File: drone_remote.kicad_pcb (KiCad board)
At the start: 2 copper layers, 151 x 78.8 mm, 92 parts, among them J1 USBC, J2 Conn_01x02_Socket, J3 UART, J4 Conn_01x05_Pin, J5 Conn_01x04_Socket, J6 Conn_01x08_Socket, J7 Conn_01x09_Socket, J8 Conn_01x09_Socket, Q1 PMOS, SW1 RST_BTN, SW2 RST_BTN, SW3 RST_BTN, SW4 RST_BTN, SW5 RST_BTN, SW6 ENC1, SW7 ENC2, U1 STM32F411RETx, U2 TC1262-33, U3 SN74ALVC14PWR, U4 SN74ALVC14PWR, U6 FT230XS, X1 8MHZ

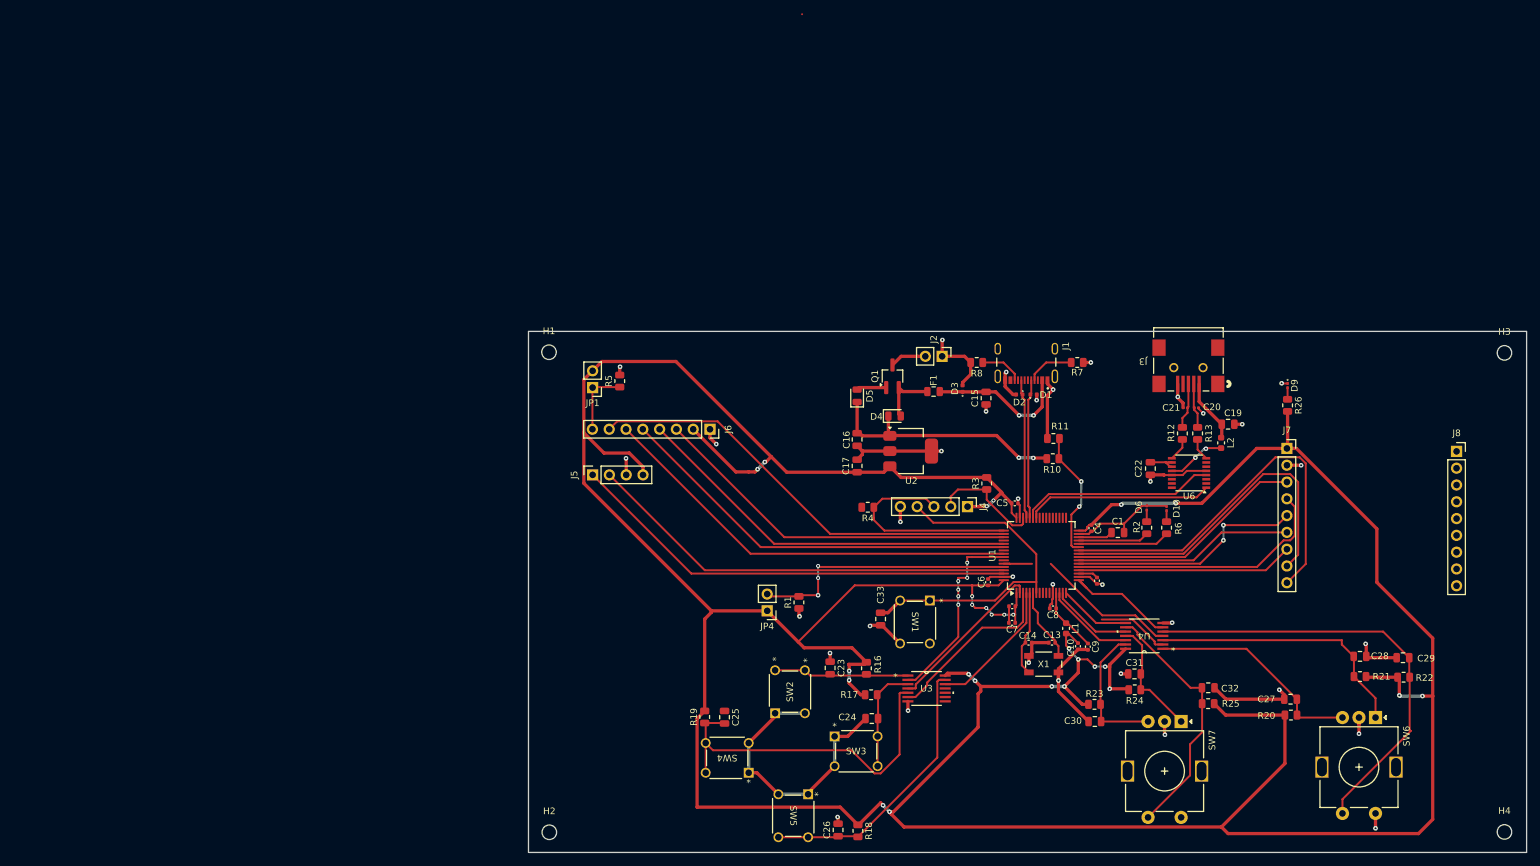
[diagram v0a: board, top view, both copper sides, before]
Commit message: updates
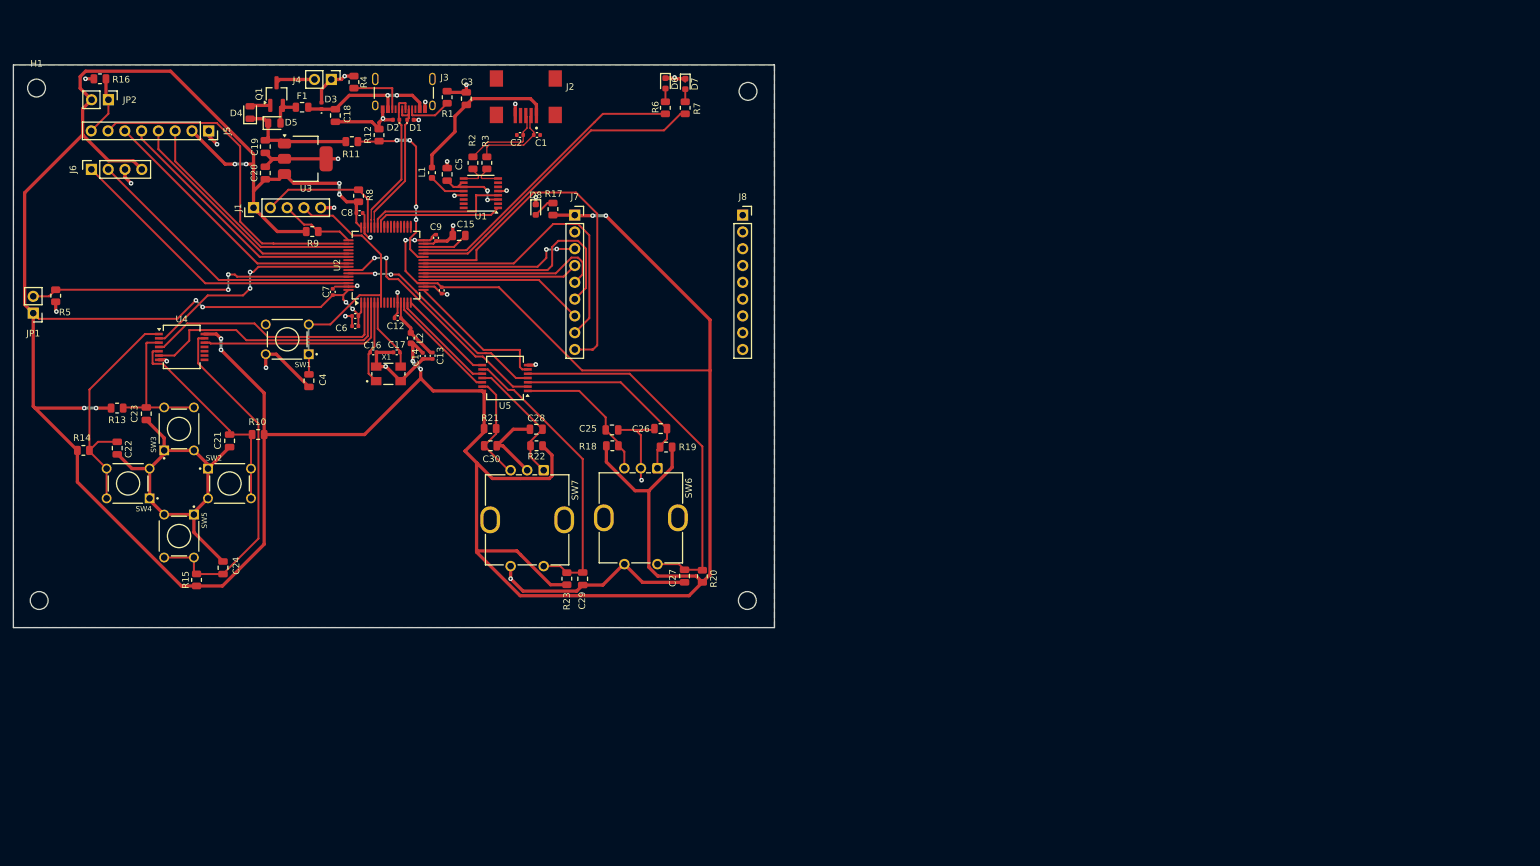
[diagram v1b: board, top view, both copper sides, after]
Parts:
- removed the J1 at (186.2, 75.9)
- added J3: GSB1C411101DS1HR, pcb_project:AMPHENOL_GSB1C411101DS1HR, F.Cu at (92.0, 35.1)
- C1: renamed from C20; footprint Capacitor_SMD:C_0201_0603Metric -> Capacitor_SMD:C_0402_1005Metric
- C2: renamed from C21; footprint Capacitor_SMD:C_0201_0603Metric -> Capacitor_SMD:C_0402_1005Metric
- D6: footprint Inductor_SMD:L_0201_0603Metric -> LED_SMD:LED_0603_1608Metric
- D7: renamed from D10; footprint Resistor_SMD:R_0201_0603Metric -> LED_SMD:LED_0603_1608Metric
- D8: renamed from D9; footprint LED_SMD:LED_0201_0603Metric -> LED_SMD:LED_0603_1608Metric
- H1, H2, H3, H4: footprint MountingHole:MountingHole_2.2mm_M2 -> MountingHole:MountingHole_2.7mm_M2.5
- J2: renamed from J3; footprint 690-005-299-043_EDA:690-005-299-043_EDA -> pcb_project:CONN5_USB1734035_NP_TEC
- SW1, SW4, SW5: footprint SW4_1825910-B_TEC:SW4_1825910-B_TEC -> pcb_project:SW_1825910-6-4
- SW2: renamed from SW3; footprint SW4_1825910-B_TEC:SW4_1825910-B_TEC -> pcb_project:SW_1825910-6-4
- SW3: renamed from SW2; footprint SW4_1825910-B_TEC:SW4_1825910-B_TEC -> pcb_project:SW_1825910-6-4
- SW6, SW7: footprint Rotary_Encoder:RotaryEncoder_Alps_EC11E-Switch_Vertical_H20mm -> Rotary_Encoder:RotaryEncoder_Bourns_Vertical_PEC12R-3x17F-Sxxxx
- U4: renamed from U3; footprint SN74ALVC14PWR:PW14 -> Package_SO:SSOP-14_5.3x6.2mm_P0.65mm
- U5: renamed from U4; footprint SN74ALVC14PWR:PW14 -> Package_SO:SSOP-14_5.3x6.2mm_P0.65mm
- X1: footprint ECS-80-10:SMD_ECS-80-10-3M-TR_ECS -> pcb_project:XTAL_ECS-80-10-30B-CWN-TR
- moved L1 126.2 mm to (96.3, 49.3)
- moved C3 125.3 mm to (101.5, 38.1), turned to -90 degrees
- moved U4 123.9 mm to (58.5, 75.7)
- moved R5 121.6 mm to (39.4, 67.9)
- moved H3 121.0 mm to (144.1, 37.0)
- moved R13 120.0 mm to (48.7, 84.9), turned to 180 degrees
- moved JP1 119.8 mm to (36.0, 70.5)
- moved H4 119.7 mm to (144.0, 114.0)
- moved R4 117.3 mm to (84.5, 35.6), turned to 90 degrees
- moved J1 117.1 mm to (69.3, 54.6), turned to 90 degrees
- moved D8 116.8 mm to (112.0, 54.9)
- moved R11 116.4 mm to (84.2, 44.6)
- moved C5 115.3 mm to (98.6, 49.5), turned to 90 degrees
- moved U1 115.2 mm to (103.7, 52.4)
- moved R3 115.0 mm to (104.6, 47.8)
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- renumbered C3 to C10, C2 to C11, C8 to C12, C9 to C13, C10 to C14, C1 to C15, C14 to C16, C13 to C17, C15 to C18, C16 to C19, C17 to C20, C24 to C21, C25 to C22, C26 to C24, C27 to C25, C28 to C26, C29 to C27, C31 to C28, C32 to C29, C19 to C3, C33 to C4, C22 to C5, C7 to C6, C6 to C7, C5 to C8, C4 to C9, D5 to D4, D4 to D5, J4 to J1, J2 to J4, J6 to J5, J5 to J6, JP4 to JP1, JP1 to JP2, L2 to L1, L1 to L2, R8 to R1, R17 to R10, R10 to R11, R11 to R12, R16 to R13, R19 to R14, R18 to R15, R5 to R16, R26 to R17, R20 to R18, R21 to R19, R12 to R2, R22 to R20, R23 to R21, R24 to R22, R25 to R23, R13 to R3, R7 to R4, R1 to R5, R2 to R6, R6 to R7, R3 to R8, R4 to R9, U6 to U1, U1 to U2, U2 to U3
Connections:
- R1 pad 1: Net-(J1-CC2) -> GND
- R1 pad 2: GND -> Net-(J3-CC1)
- R8 pad 1: /SWDIO -> +3.3V
- R8 pad 2: +3.3V -> /SWDIO
- R9 pad 1: /SWCLK -> +3.3V
- R9 pad 2: +3.3V -> /SWCLK
- U4 pad 1: /SW2 -> /SW4
- U4 pad 3: /SW3 -> /SW2
- U4 pad 5: /SW4 -> /SW3
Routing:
- net /MCU_LED: track 13.9 -> 48.3 mm
- net /HB_LED: track 10.7 -> 45.1 mm
- net /TIM4_CH1: track 11.0 -> 37.6 mm, vias 0 -> 2
- net /ST7735_DC: track 64.9 -> 42.1 mm
- net /I2C1_SCL: track 65.6 -> 43.3 mm
- net /I2C1_SDA: track 68.4 -> 46.0 mm
- net /ST7735_nRST: track 62.0 -> 39.9 mm
- net /SPI3_MOSI: track 59.2 -> 38.1 mm
- net /SWCLK: track 32.4 -> 11.3 mm
- net /SPI3_SCK: track 56.3 -> 36.2 mm
- net /REG_IN: track 38.1 -> 18.3 mm, vias 2 -> 0
- net GND: track 210.1 -> 228.2 mm, vias 35 -> 29
- net /SW4: track 53.6 -> 36.2 mm
- net /SPI1_SCK: track 40.7 -> 23.6 mm
- net /SPI3_nCS: track 67.2 -> 51.1 mm
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- added copper zone on B.Cu, net GND
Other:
- board size 151 x 78.8 mm -> 115.1 x 85.1 mm
